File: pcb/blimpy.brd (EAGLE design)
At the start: 70 x 70 mm, 74 parts, among them J4 3-PIN SMD, J5 3-PIN SMD, J6 3-PIN SMD, J7 3-PIN SMD, Q1 mmbt2222, Q2 mmbt2222, Q3 DMG3415U, U1 RGB, U10 MAX17048, U2 AP2112-3.3, U3 MCP73831T-2, U4 BNO080, U5 SX1509, U6 SX1509, U7 CP2104, U9 ESP-WROOM-32

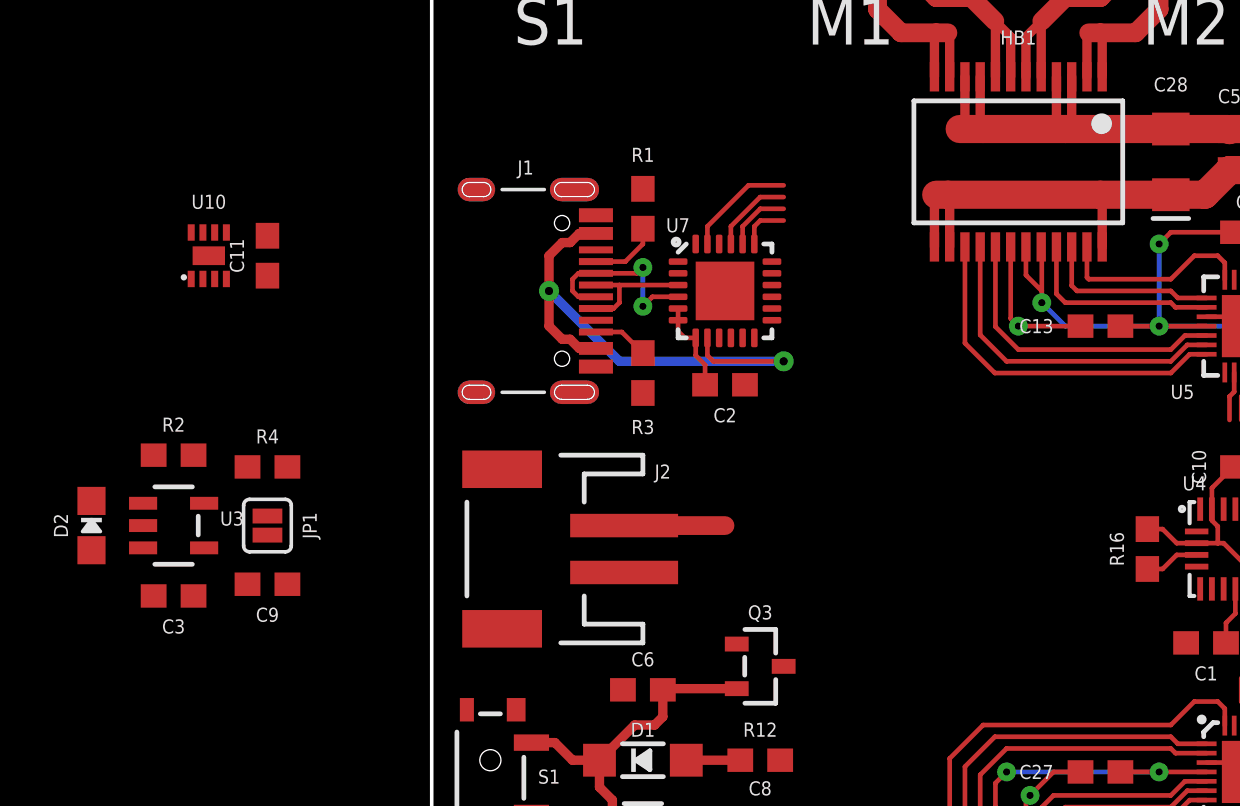
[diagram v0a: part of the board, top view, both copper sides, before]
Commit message: more traces
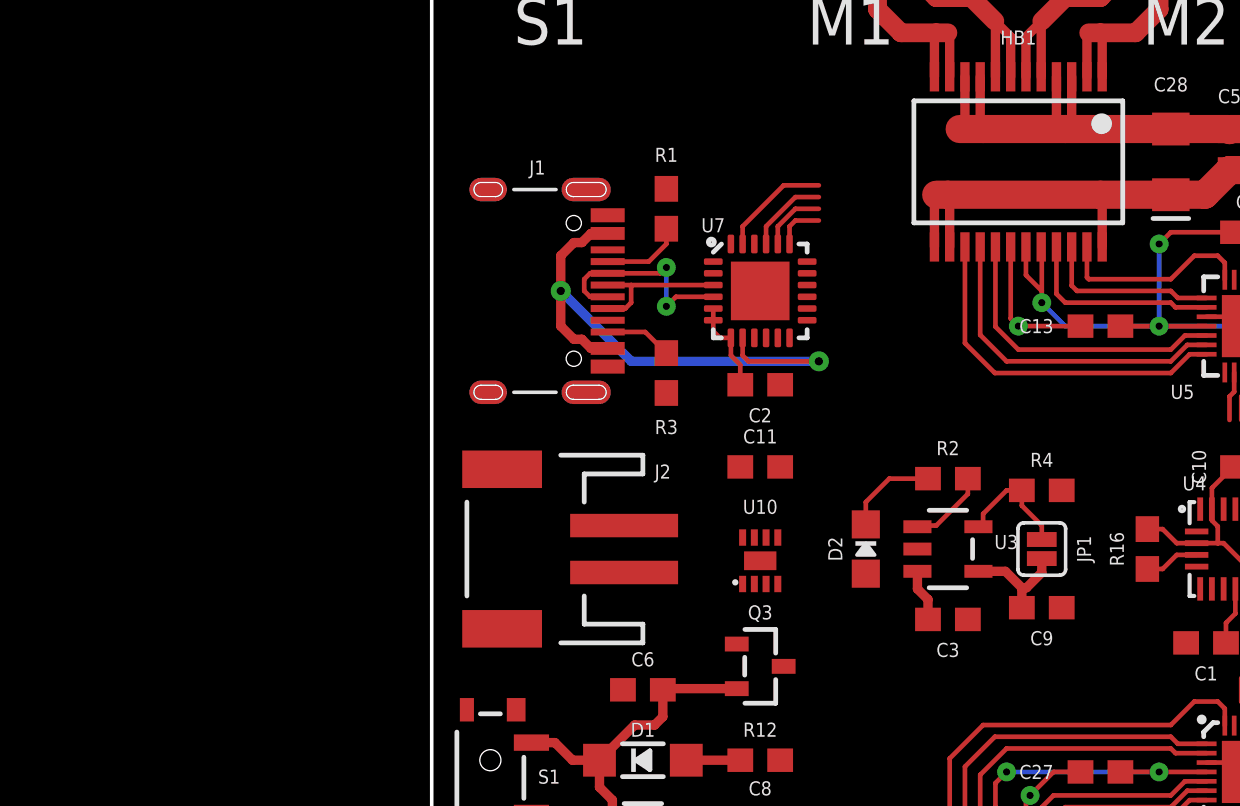
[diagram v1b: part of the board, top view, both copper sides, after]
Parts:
- moved C3 33.0 mm to (22.0, 32.0)
- moved C9 33.0 mm to (26.0, 32.5)
- moved D2 33.0 mm to (18.5, 35.0)
- moved JP1 33.0 mm to (26.0, 35.0)
- moved R2 33.0 mm to (22.0, 38.0)
- moved R4 33.0 mm to (26.0, 37.5)
- moved U3 33.0 mm to (22.0, 35.0)
- moved U10 26.9 mm to (14.0, 34.5)
- moved C11 22.8 mm to (14.0, 38.5), turned to 0 degrees
- moved C2 1.50 mm to (14.0, 42.0)
- moved U7 1.50 mm to (14.0, 46.0)
- moved R1 1.00 mm to (10.0, 49.5)
- moved R3 1.00 mm to (10.0, 42.5)
- moved J1 0.50 mm to (7.50, 46.0)
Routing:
- net V_USB: track 25.7 -> 31.4 mm
- net N$4: track 0.00 -> 5.14 mm
- net N$1: track 0.00 -> 4.01 mm
- net N$3: track 0.00 -> 3.38 mm
- net V_BATT: track 87.2 -> 85.1 mm
- net N$6: track 8.14 -> 9.14 mm
- net N$2: track 5.35 -> 6.35 mm
- net N$5: track 2.96 -> 3.46 mm
- net N$17: track 2.37 -> 2.87 mm
